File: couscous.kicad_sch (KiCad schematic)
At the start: 141 parts, among them SW1 SW_PUSH, SW10 SW_PUSH, SW11 SW_PUSH, SW12 SW_PUSH, SW13 SW_PUSH, SW14 SW_PUSH, SW15 SW_PUSH, SW16 SW_PUSH, SW17 SW_PUSH, SW18 SW_PUSH, SW19 SW_PUSH, SW2 SW_PUSH, SW20 SW_PUSH, SW21 SW_PUSH, SW22 SW_PUSH, SW23 SW_PUSH, SW24 SW_PUSH, SW25 SW_PUSH, SW26 SW_PUSH, SW27 SW_PUSH, SW28 SW_PUSH, SW29 SW_PUSH, SW3 SW_PUSH, SW30 SW_PUSH, SW31 SW_PUSH, SW32 SW_PUSH, SW33 SW_PUSH, SW34 SW_PUSH, SW35 SW_PUSH, SW36 SW_PUSH, SW37 SW_PUSH, SW38 SW_PUSH, SW39 SW_PUSH, SW4 SW_PUSH, SW40 SW_PUSH, SW41 SW_PUSH, SW42 SW_PUSH, SW43 SW_PUSH, SW44 SW_PUSH, SW45 SW_PUSH, SW46 SW_PUSH, SW47 SW_PUSH, SW48 SW_PUSH, SW49 SW_PUSH, SW5 SW_PUSH, SW50 SW_PUSH, SW51 SW_PUSH, SW52 SW_PUSH, SW53 SW_PUSH, SW54 SW_PUSH, SW55 SW_PUSH, SW56 SW_PUSH, SW57 SW_PUSH, SW58 SW_PUSH, SW59 SW_PUSH, SW6 SW_PUSH, SW60 SW_PUSH, SW61 SW_SPST, SW62 SW_SPST, SW63 SW_SPST, SW64 SW_SPST, SW65 SW_SPST, SW7 SW_PUSH, SW8 SW_PUSH, SW9 SW_PUSH, U1 SeeeduinoXIAO

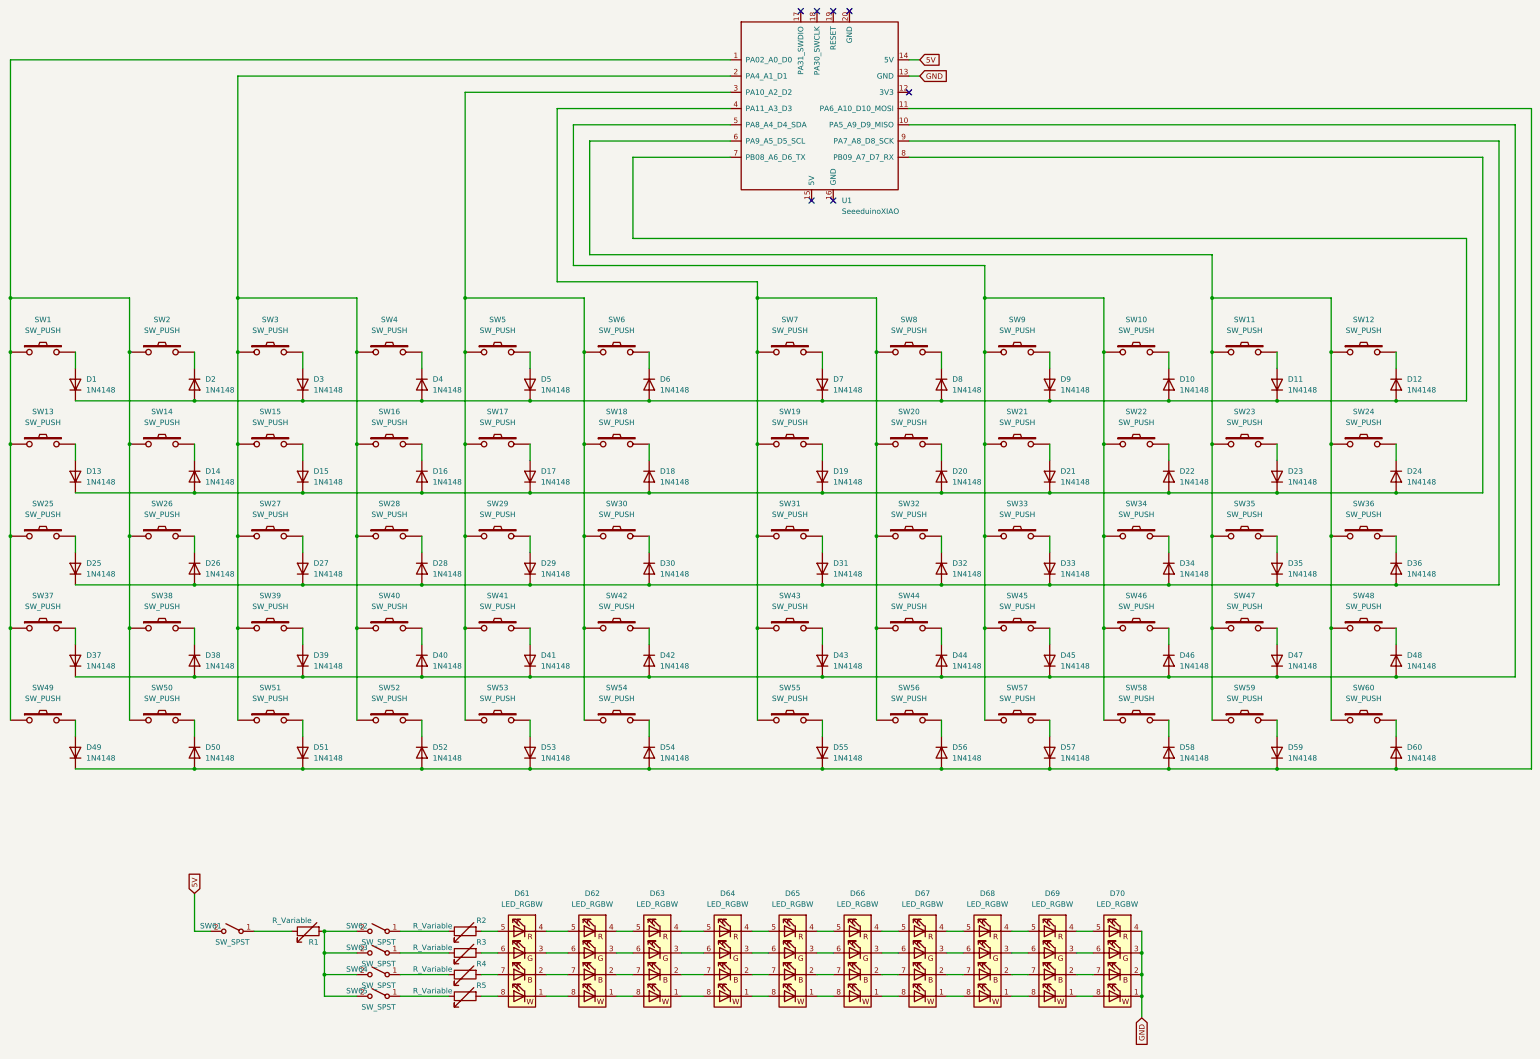
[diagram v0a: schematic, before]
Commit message: Routing!
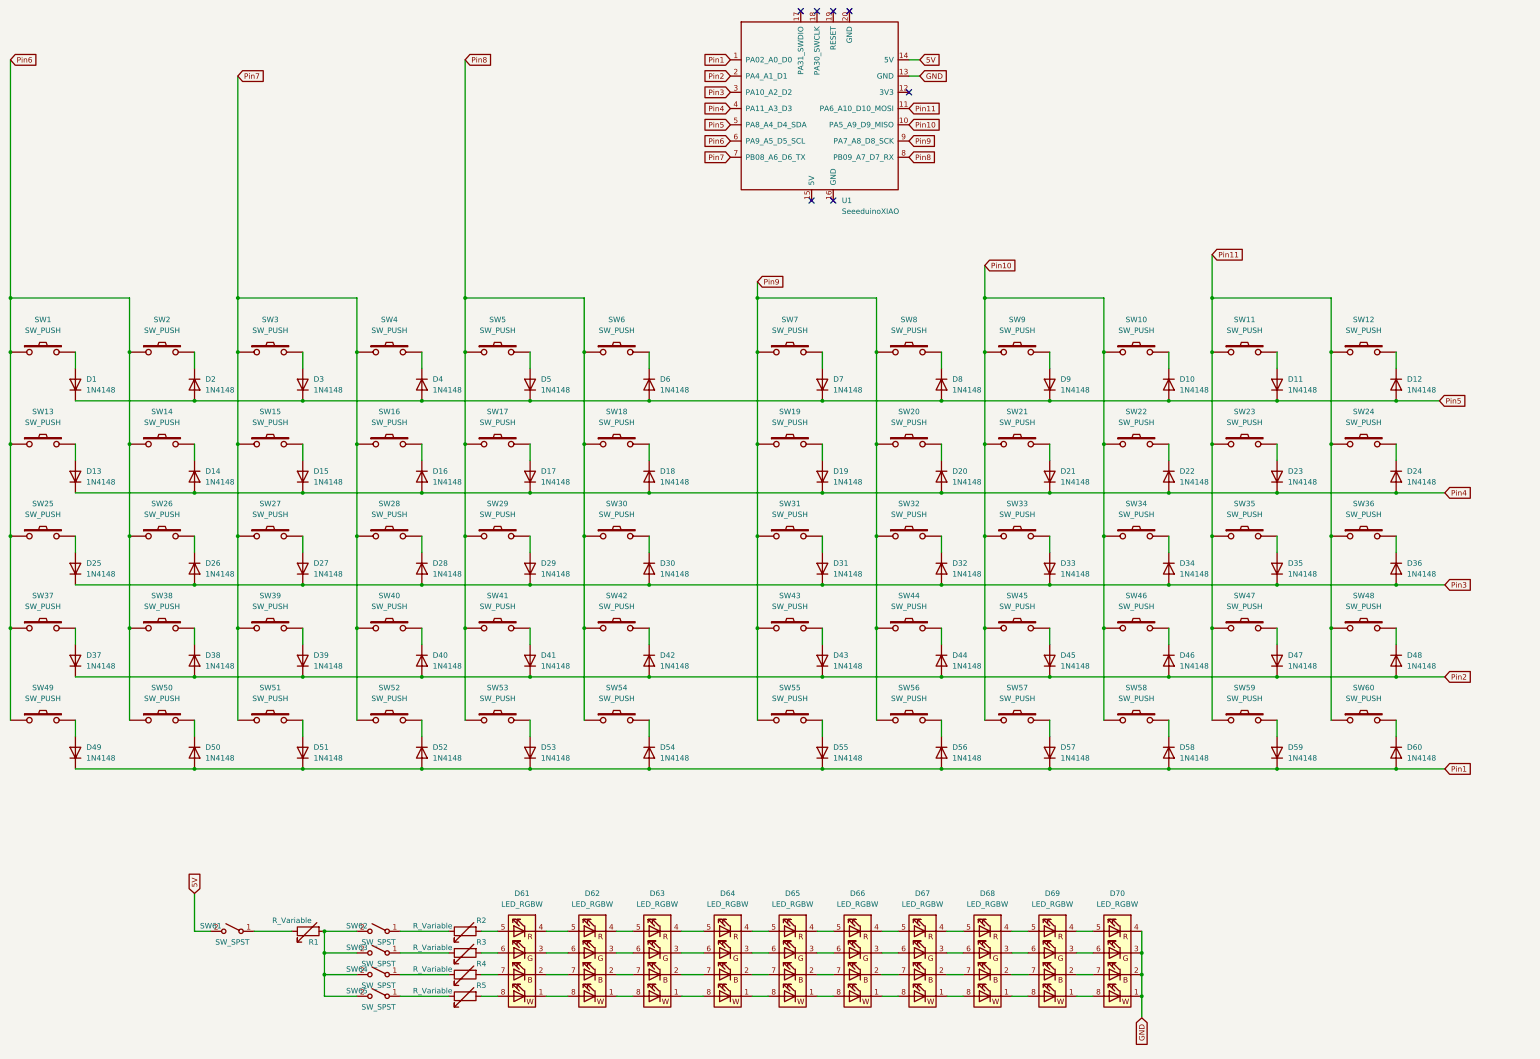
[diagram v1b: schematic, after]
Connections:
- net Pin3: now reaches D25.1 (K), D26.2 (A), D27.1 (K), D28.2 (A), D29.1 (K), D30.2 (A), D31.1 (K), D32.2 (A), D33.1 (K), D34.2 (A), D35.1 (K), D36.2 (A)
- net Pin3: now also U1.3 (PA10_A2_D2); no longer U1.9 (PA7_A8_D8_SCK)
- net Pin8: now reaches SW17.1, SW18.1, SW29.1, SW30.1, SW41.1, SW42.1, SW5.1, SW53.1, SW54.1, SW6.1
- net Pin8: now also U1.8 (PB09_A7_D7_RX); no longer U1.3 (PA10_A2_D2)
- net Pin10: now reaches SW10.1, SW21.1, SW22.1, SW33.1, SW34.1, SW45.1, SW46.1, SW57.1, SW58.1, SW9.1
- net Pin10: now also U1.10 (PA5_A9_D9_MISO); no longer U1.5 (PA8_A4_D4_SDA)
- net Pin6: now reaches SW1.1, SW13.1, SW14.1, SW2.1, SW25.1, SW26.1, SW37.1, SW38.1, SW49.1, SW50.1
- net Pin6: now also U1.6 (PA9_A5_D5_SCL); no longer U1.1 (PA02_A0_D0)
- net Pin1: now reaches D49.1 (K), D50.2 (A), D51.1 (K), D52.2 (A), D53.1 (K), D54.2 (A), D55.1 (K), D56.2 (A), D57.1 (K), D58.2 (A), D59.1 (K), D60.2 (A)
- net Pin1: now also U1.1 (PA02_A0_D0); no longer U1.11 (PA6_A10_D10_MOSI)
- net Pin9: now reaches SW19.1, SW20.1, SW31.1, SW32.1, SW43.1, SW44.1, SW55.1, SW56.1, SW7.1, SW8.1
- net Pin9: now also U1.9 (PA7_A8_D8_SCK); no longer U1.4 (PA11_A3_D3)
- net Pin5: now reaches D1.1 (K), D10.2 (A), D11.1 (K), D12.2 (A), D2.2 (A), D3.1 (K), D4.2 (A), D5.1 (K), D6.2 (A), D7.1 (K), D8.2 (A), D9.1 (K)
- net Pin5: now also U1.5 (PA8_A4_D4_SDA); no longer U1.7 (PB08_A6_D6_TX)
- net Pin2: now reaches D37.1 (K), D38.2 (A), D39.1 (K), D40.2 (A), D41.1 (K), D42.2 (A), D43.1 (K), D44.2 (A), D45.1 (K), D46.2 (A), D47.1 (K), D48.2 (A)
- net Pin2: now also U1.2 (PA4_A1_D1); no longer U1.10 (PA5_A9_D9_MISO)
- net Pin7: now reaches SW15.1, SW16.1, SW27.1, SW28.1, SW3.1, SW39.1, SW4.1, SW40.1, SW51.1, SW52.1
- net Pin7: now also U1.7 (PB08_A6_D6_TX); no longer U1.2 (PA4_A1_D1)
- net Pin4: now reaches D13.1 (K), D14.2 (A), D15.1 (K), D16.2 (A), D17.1 (K), D18.2 (A), D19.1 (K), D20.2 (A), D21.1 (K), D22.2 (A), D23.1 (K), D24.2 (A)
- net Pin4: now also U1.4 (PA11_A3_D3); no longer U1.8 (PB09_A7_D7_RX)
- net Pin11: now reaches SW11.1, SW12.1, SW23.1, SW24.1, SW35.1, SW36.1, SW47.1, SW48.1, SW59.1, SW60.1
- net Pin11: now also U1.11 (PA6_A10_D10_MOSI); no longer U1.6 (PA9_A5_D5_SCL)
